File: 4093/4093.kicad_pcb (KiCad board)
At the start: 2 copper layers, 12 parts, among them J1 Screw_Terminal_01x02, U1 HEF4093B

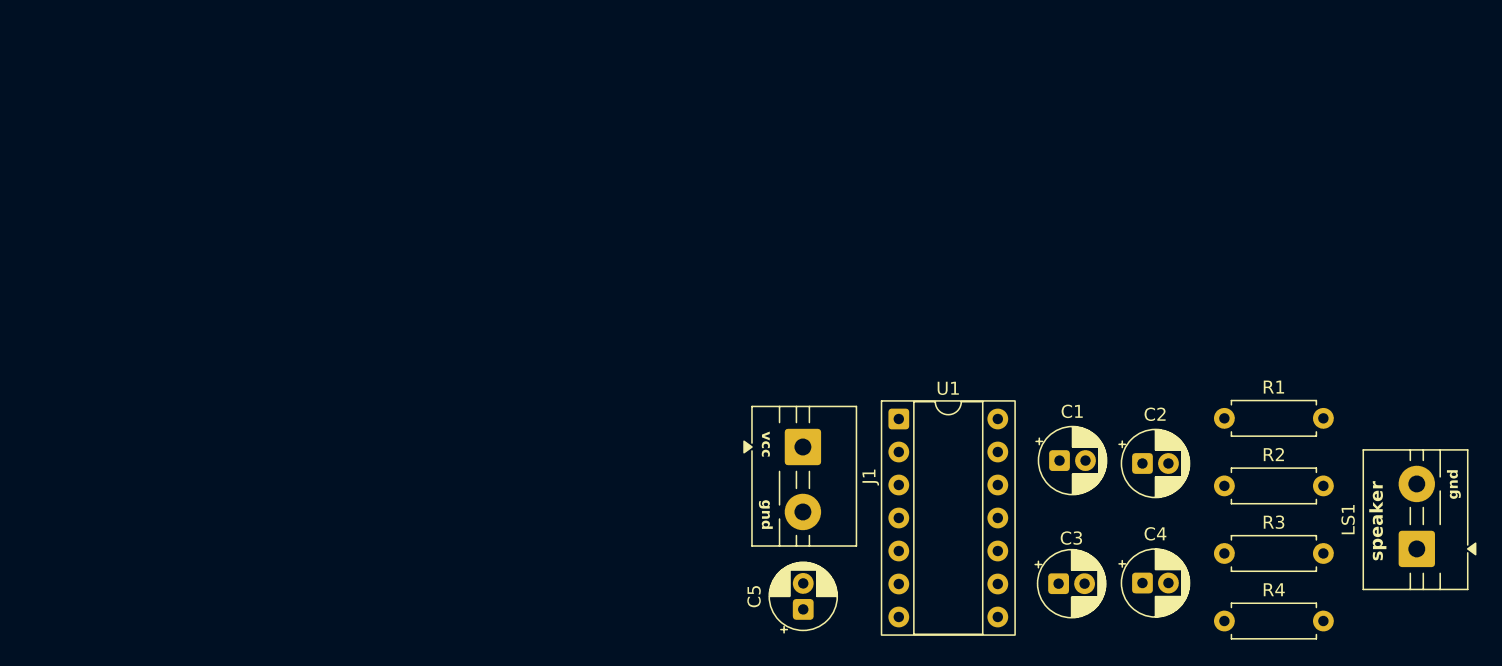
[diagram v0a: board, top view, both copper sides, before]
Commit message: gerbers + correcciones
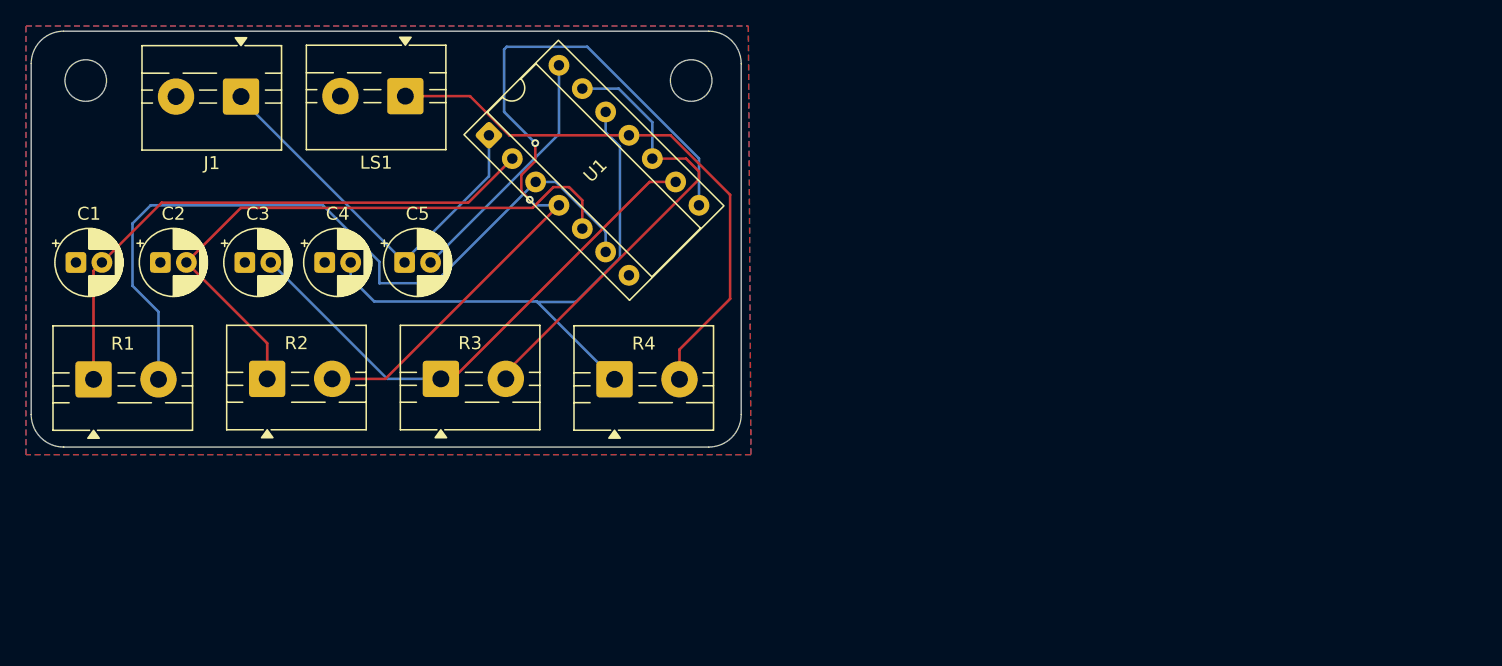
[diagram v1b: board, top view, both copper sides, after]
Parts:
- added H1: MountingHole, MountingHole:MountingHole_3.2mm_M3, F.Cu at (137.4, 57.0)
- added H2: MountingHole, MountingHole:MountingHole_3.2mm_M3, F.Cu at (90.8, 57.0)
- R1, R2, R3, R4: footprint Resistor_THT:R_Axial_DIN0207_L6.3mm_D2.5mm_P7.62mm_Horizontal -> TerminalBlock:TerminalBlock_MaiXu_MX126-5.0-02P_1x02_P5.00mm
- moved R1 87.1 mm to (91.4, 80.0)
- moved LS1 85.3 mm to (115.4, 58.2), turned to 180 degrees
- moved C1 77.2 mm to (90.0, 71.0)
- moved C2 77.2 mm to (96.5, 71.0)
- moved R2 74.1 mm to (104.8, 80.0)
- moved C4 67.6 mm to (109.2, 71.0)
- moved C3 67.3 mm to (103.0, 71.0)
- moved R3 61.8 mm to (118.1, 80.0)
- moved J1 51.0 mm to (102.8, 58.2), turned to 180 degrees
- moved R4 50.5 mm to (131.5, 80.0)
- moved C5 40.7 mm to (115.3, 71.0), turned to 0 degrees
- moved U1 38.4 mm to (121.8, 61.2), turned to 45 degrees
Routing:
- net Net-(R2-Pad2): track 0.00 -> 60.9 mm, vias 0 -> 2
- net Net-(R1-Pad2): track 0.00 -> 59.7 mm
- net Net-(C2-Pad2): track 0.00 -> 47.0 mm
- net Net-(C4-Pad2): track 0.00 -> 44.2 mm
- net Net-(C1-Pad2): track 0.00 -> 44.2 mm
- net Net-(LS1-Pad1): track 0.00 -> 44.0 mm
- net Net-(C3-Pad2): track 0.00 -> 41.1 mm
- net Net-(R3-Pad2): track 0.00 -> 35.4 mm
- net VCC: track 0.00 -> 30.5 mm
- net Net-(U1E-VCC): track 0.00 -> 19.3 mm
- added copper zone on B.Cu, net GND
- added copper zone on F.Cu, net GND
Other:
- board outline added: 54.7 x 32 mm
- board text removed: "gnd"
- board text removed: "speaker"
- board text removed: "vcc"

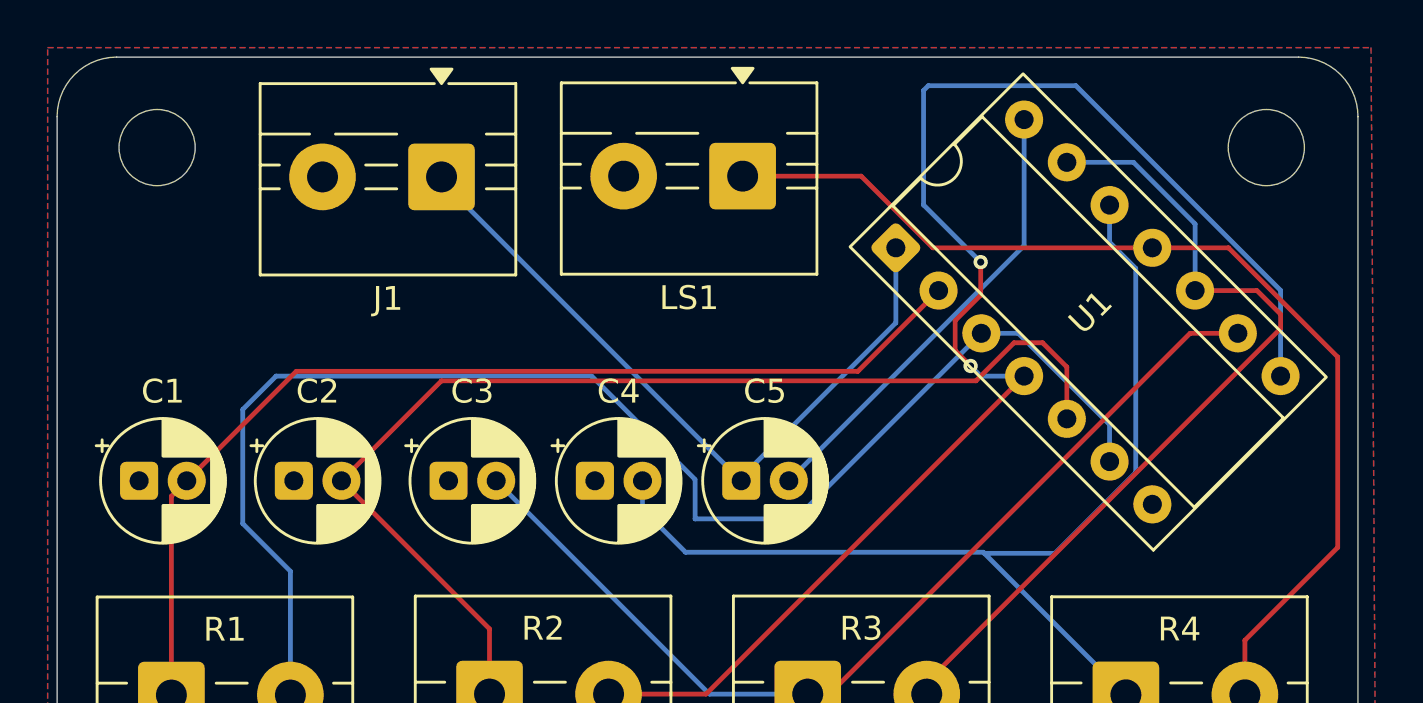
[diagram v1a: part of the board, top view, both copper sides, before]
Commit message: actualizar gerber
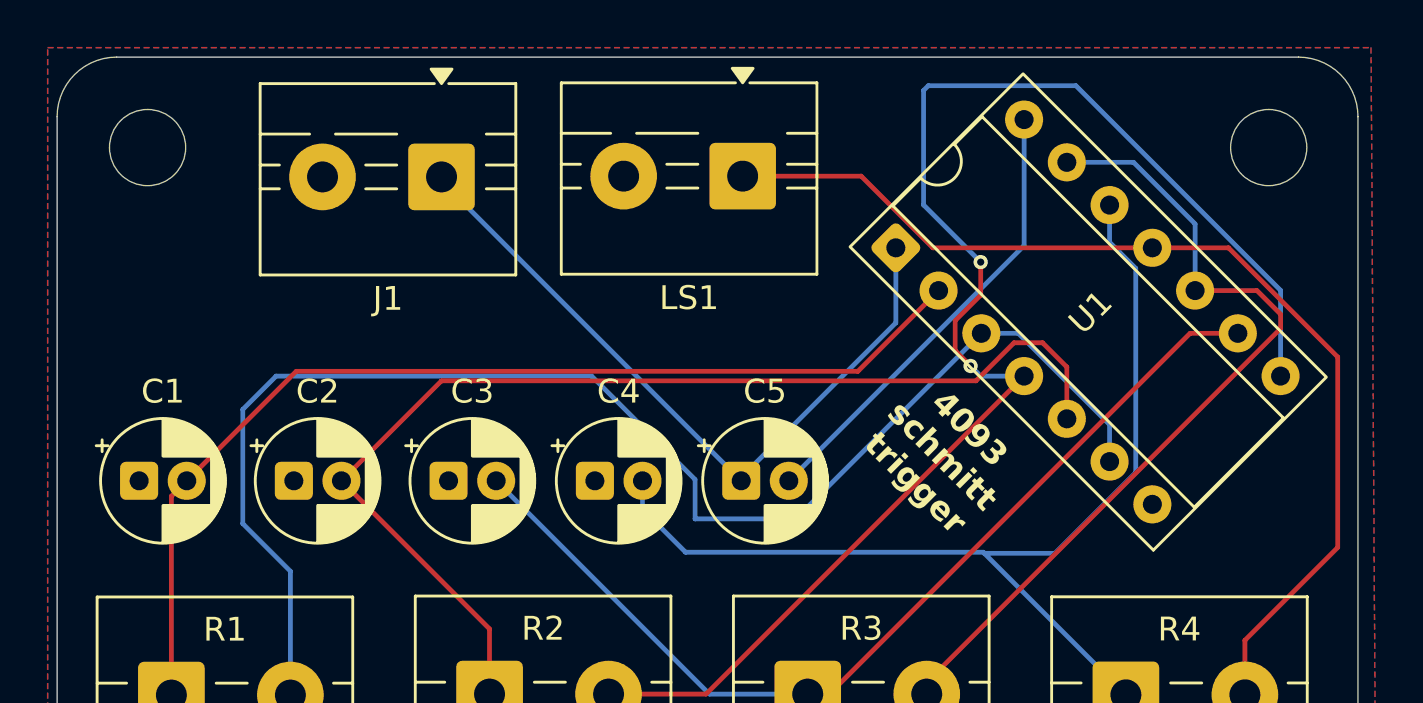
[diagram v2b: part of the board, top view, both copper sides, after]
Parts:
- moved H1 47.0 mm to (90.4, 57.0)
- moved H2 46.7 mm to (137.5, 57.0)
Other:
- board text added: "4093 schmitt trigger"
